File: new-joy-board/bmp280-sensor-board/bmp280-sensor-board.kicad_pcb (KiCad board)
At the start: 2 copper layers, 26.1 x 31.1 mm, 16 parts, among them J1 Conn_01x05, U1 TPS76933, U2 bmp280-board, U3 P82B715, U4 MPU6050_Breakout

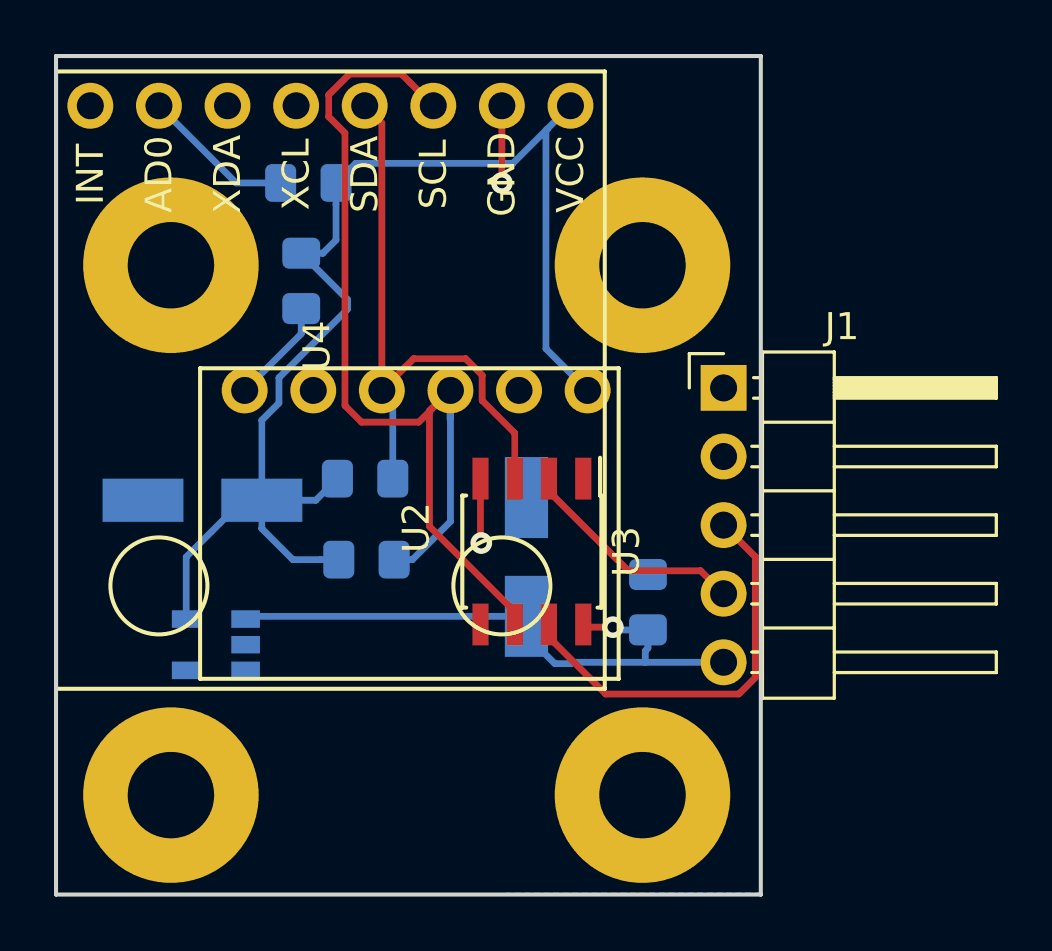
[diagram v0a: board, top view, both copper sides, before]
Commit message: Continue work on daughter board
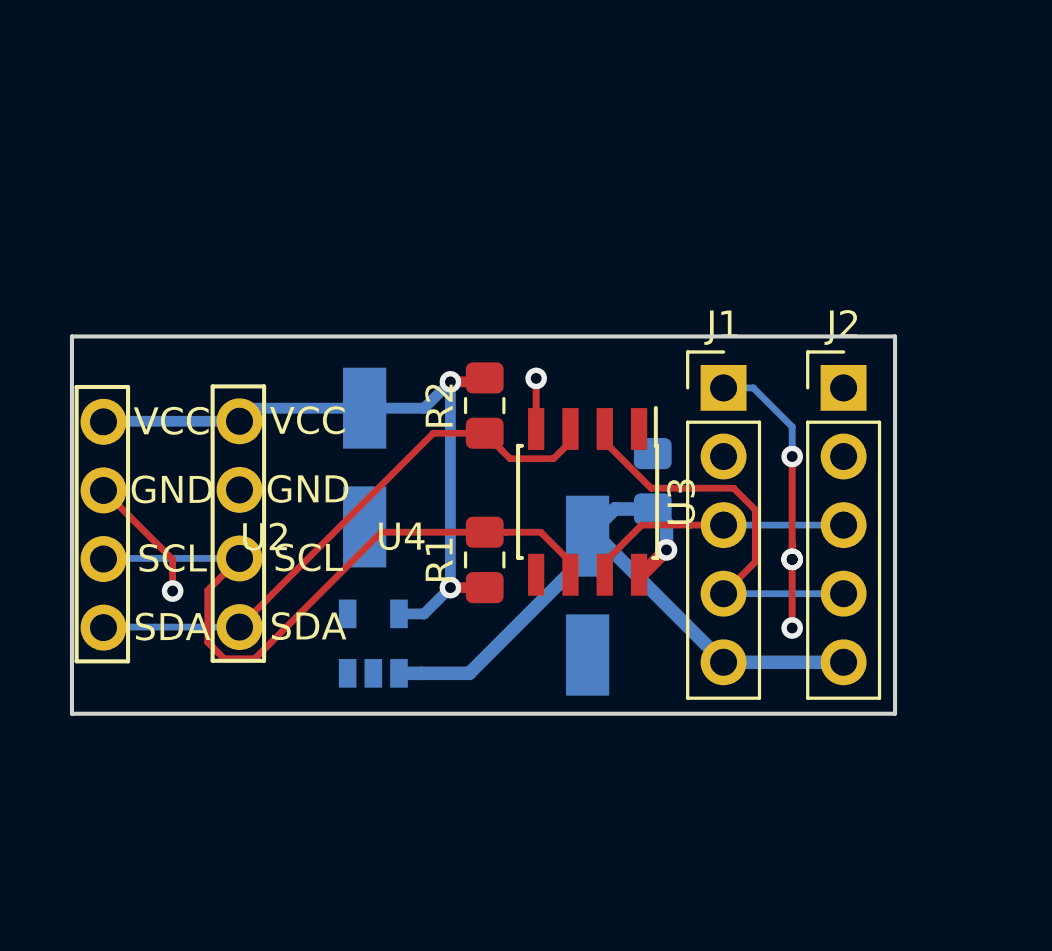
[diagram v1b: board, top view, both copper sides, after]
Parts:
- removed R3, R4: 0K, Resistor_SMD:R_0805_2012Metric_Pad1.15x1.40mm_HandSolder
- removed REF** (x4): VAL**, new-joy:z_MountPTH_3mm
- added J2: Conn_01x05, Connector_PinHeader_2.54mm:PinHeader_1x05_P2.54mm_Vertical, F.Cu at (123.1, 44.0)
- J1: footprint Connector_PinHeader_2.54mm:PinHeader_1x05_P2.54mm_Horizontal -> Connector_PinHeader_2.54mm:PinHeader_1x05_P2.54mm_Vertical
- R1, R2: moved to F.Cu
- U2: value bmp280-board -> generic-i2c-device; footprint new-joy:bmp280-board-footprint -> new-joy:generic-i2c-device
- U4: value MPU6050_Breakout -> generic-i2c-device; footprint new-joy:MPU6050_Breakout -> new-joy:generic-i2c-device
- moved U4 7.09 mm to (106.8, 49.1), turned to 0 degrees
- moved C2 6.13 mm to (105.4, 47.0), turned to 270 degrees
- moved U1 5.83 mm to (105.7, 53.5), turned to 90 degrees
- moved U2 5.59 mm to (101.7, 49.1), turned to 0 degrees
- moved R2 5.19 mm to (109.9, 44.7), turned to 90 degrees
- moved C3 4.48 mm to (116.1, 47.5)
- moved R1 4.38 mm to (109.9, 50.4), turned to 90 degrees
- moved U3 2.77 mm to (113.7, 48.3)
- moved C1 2.68 mm to (113.7, 51.7), turned to 270 degrees
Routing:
- net +3V3: track 48.5 -> 26.0 mm, vias 0 -> 2
- net /SCL: track 40.0 -> 25.2 mm
- net GND: track 5.26 -> 17.9 mm, vias 2 -> 6
- net /SDABUF: track 8.51 -> 15.1 mm
- net Net-(R3-Pad1): track 5.69 -> 0.00 mm
- net /SCLBUF: track 15.4 -> 9.89 mm
- net +5V: track 22.6 -> 26.9 mm
- net Net-(R4-Pad2): track 3.90 -> 0.00 mm
- net /SDA: track 23.6 -> 21.4 mm
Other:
- board size 26.1 x 31.1 mm -> 30.5 x 14 mm
- net class 3.3V added: clearance 0.2, trace_width 0.4, via_dia 0.8, via_drill 0.4
- net class 5V added: clearance 0.2, trace_width 0.5, via_dia 0.8, via_drill 0.4
